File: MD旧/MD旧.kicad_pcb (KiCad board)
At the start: 2 copper layers, 42 parts, among them J1 Conn_01x04_Pin, J2 Conn_02x04_Odd_Even, J3 XT60-M, J4 XT60-M

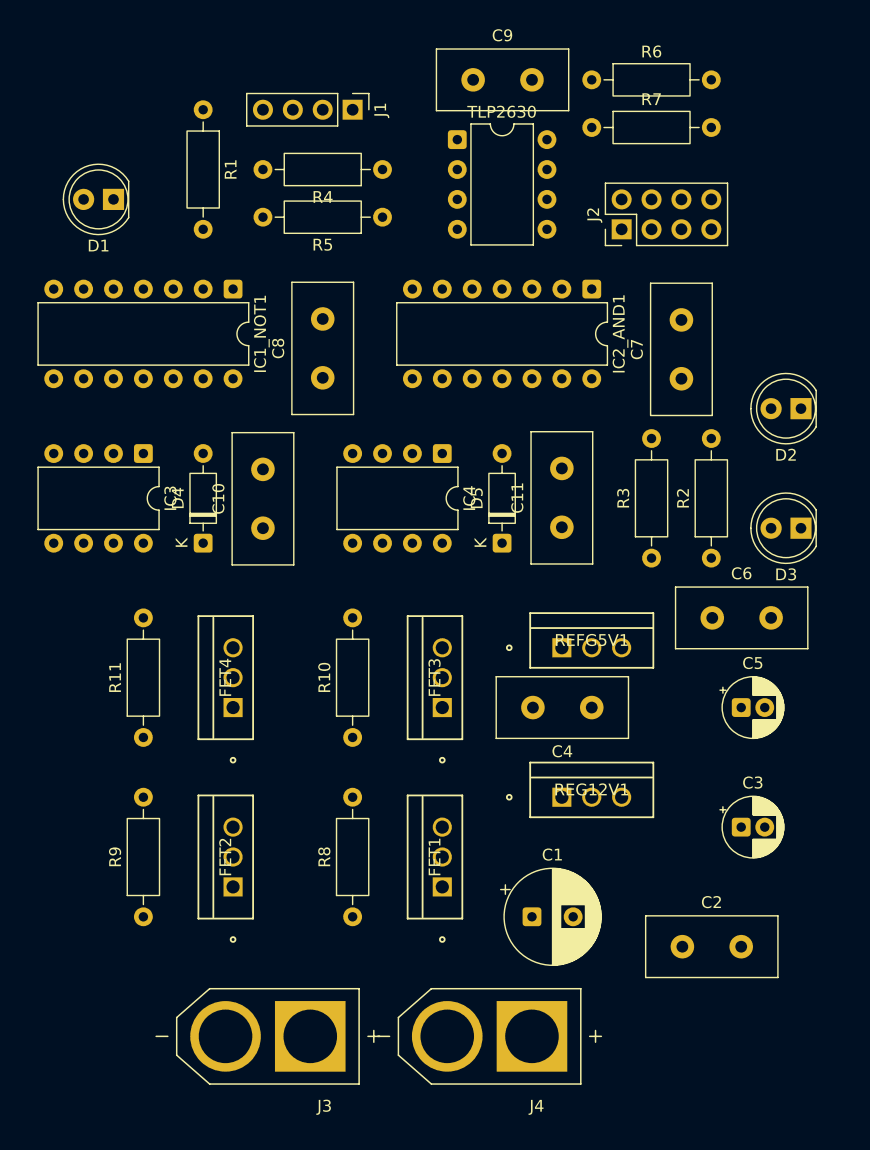
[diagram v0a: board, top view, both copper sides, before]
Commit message: 配線できたよー
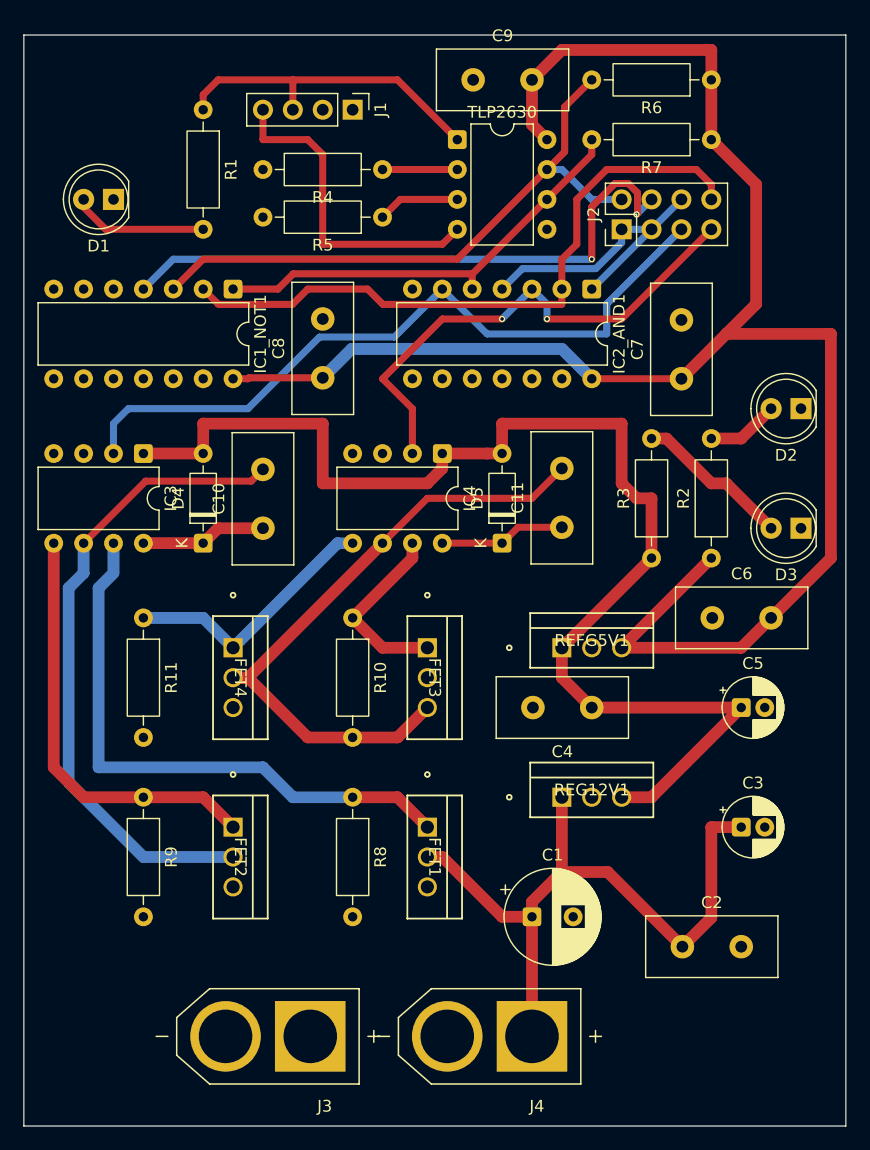
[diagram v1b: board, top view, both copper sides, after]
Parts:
- moved R7 10.2 mm to (167.6, 66.0), turned to 180 degrees
- moved R8 10.2 mm to (137.2, 121.9), turned to -90 degrees
- moved R9 10.2 mm to (119.4, 121.9), turned to -90 degrees
- moved R10 10.2 mm to (137.2, 106.7), turned to -90 degrees
- moved R11 10.2 mm to (119.4, 106.7), turned to -90 degrees
- moved R6 10.2 mm to (167.6, 61.0), turned to 180 degrees
- moved FET1 5.24 mm to (143.5, 124.5), turned to -90 degrees
- moved FET3 5.24 mm to (143.5, 109.2), turned to -90 degrees
- moved FET2 5.08 mm to (127.0, 124.5), turned to -90 degrees
- moved FET4 5.08 mm to (127.0, 109.2), turned to -90 degrees
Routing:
- net +2V5: track 0.00 -> 153.9 mm
- net MC: track 0.00 -> 110.3 mm
- net +12V: track 0.00 -> 108.7 mm
- net GATE1: track 0.00 -> 62.3 mm
- net +24V: track 0.00 -> 59.0 mm
- net DIGITAL: track 0.00 -> 55.8 mm
- net PWM_NOT: track 0.00 -> 52.6 mm
- net PWM1: track 0.00 -> 52.3 mm, vias 0 -> 2
- net Net-(FET1-G): track 0.00 -> 49.6 mm
- net GATE2: track 0.00 -> 43.5 mm, vias 0 -> 2
- net DIGITAL_NOT: track 0.00 -> 37.8 mm
- net Net-(FET2-G): track 0.00 -> 36.4 mm
- net PWM_IN: track 0.00 -> 28.0 mm
- net DIGITAL_IN: track 0.00 -> 27.7 mm
- net PWM2: track 0.00 -> 26.2 mm
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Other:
- board outline added: 69.8 x 92.7 mm
